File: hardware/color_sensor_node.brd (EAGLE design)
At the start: 27.9 x 27.9 mm, 20 parts, among them J1 JTAG, J2 JTAG, U1 ISL29125, U2 3.3V, U3 WS2811

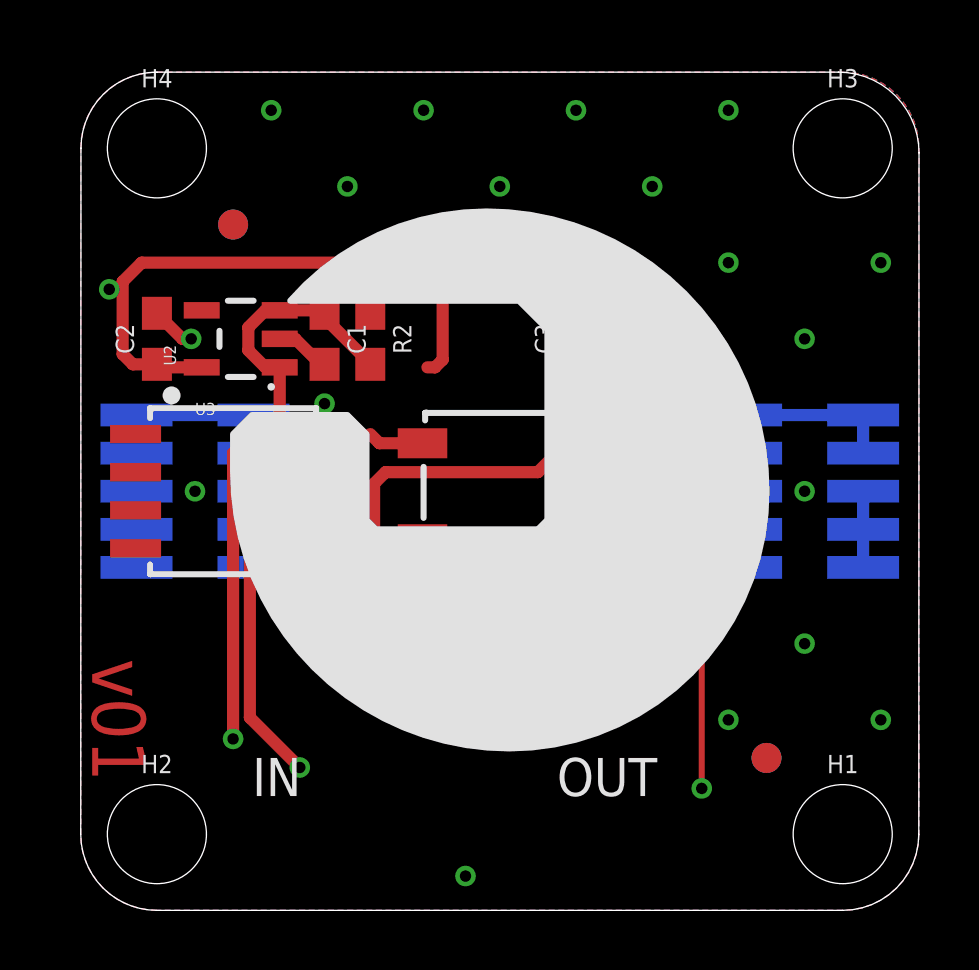
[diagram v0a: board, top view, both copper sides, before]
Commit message: idk
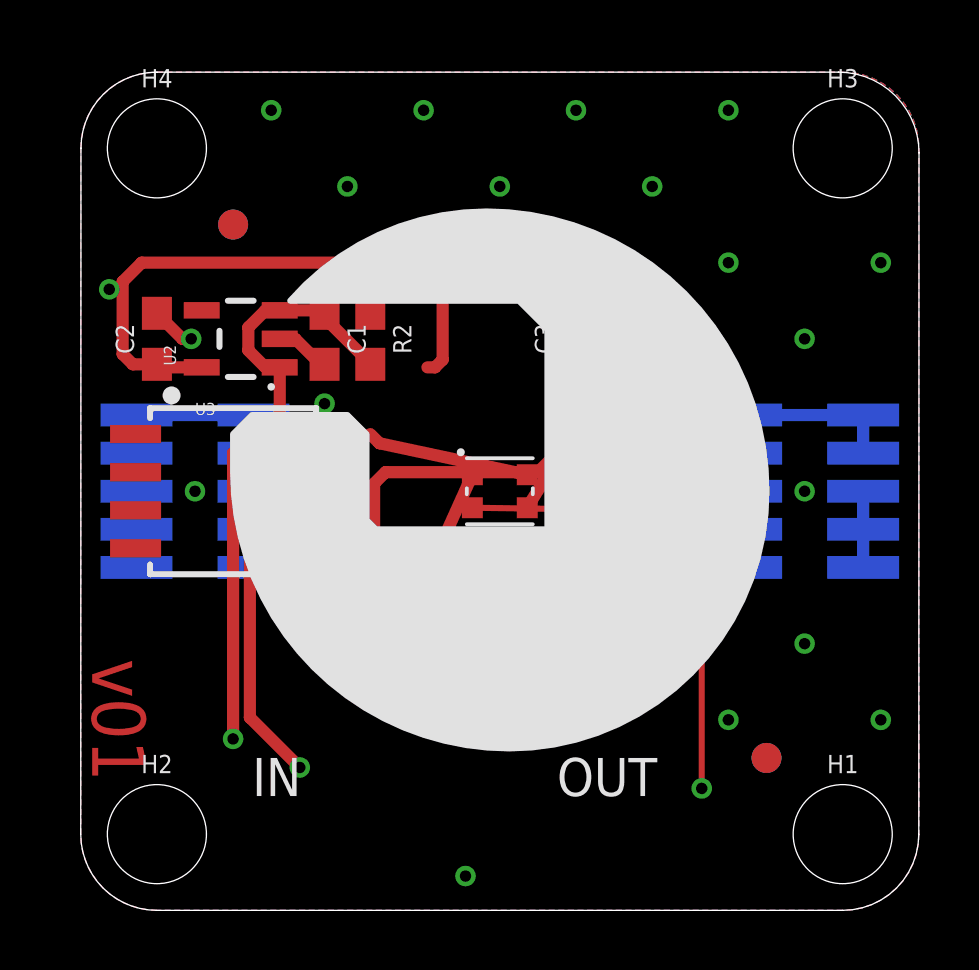
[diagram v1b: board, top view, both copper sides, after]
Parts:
- D1: device SparkFun-LED:WS2812B -> SparkFun-LED:WS2812-2020
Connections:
- net 5V: now also D1.4; no longer D1.1
- net DOUT: now also D1.1; no longer D1.2
- net GND: now also D1.2; no longer D1.3
- net N$4: now also D1.3; no longer D1.4
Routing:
- net 5V: track 27.7 -> 31.3 mm
- net DOUT: track 1.54 -> 4.05 mm
- net GND: track 16.5 -> 19.0 mm
- net N$4: track 10.7 -> 12.9 mm
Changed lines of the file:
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@@
 <attribute name="VALUE" x="3.302" y="19.05" size="0.6096" layer="27" font="vector" ratio="20" rot="R90" align="top-center"/>
 </element>
-<element name="D1" library="SparkFun-LED" package="WS2812B" value="WS2812B" x="13.97" y="13.97" rot="R180">
-<attribute name="PROD_ID" value="DIO-12503" x="13.97" y="13.97" size="1.778" layer="27" rot="R180" display="off"/>
-<attribute name="VALUE" value="WS2812B" x="13.97" y="13.97" size="1.778" layer="27" rot="R180" display="off"/>
+<element name="D1" library="SparkFun-LED" package="WS2812-2020" value="WS2812B" x="13.97" y="13.97" rot="R180">
 <attribute name="VALUE" x="13.97" y="16.764" size="0.6096" layer="27" font="vector" ratio="20" rot="R180" align="top-center"/>
 </element>
@@
 <contactref element="U1" pad="3"/>
 <contactref element="U3" pad="4"/>
-<contactref element="D1" pad="3"/>
+<contactref element="D1" pad="2"/>
 <wire x1="7.151" y1="19.05" x2="6.6341" y2="19.05" width="0.4064" layer="1"/>
 <wire x1="8.128" y1="18.2" x2="8.001" y2="18.2" width="0.4064" layer="1"/>
@@
 <via x="19.05" y="11.43" extent="1-16" drill="0.381"/>
 <wire x1="18.33" y1="13.47" x2="16.645" y2="13.47" width="0.2032" layer="1"/>
-<wire x1="16.547" y1="13.372" x2="16.547" y2="12.37" width="0.2032" layer="1"/>
+<wire x1="16.547" y1="13.372" x2="13.055" y2="13.42" width="0.2032" layer="1"/>
 <wire x1="16.645" y1="13.47" x2="16.547" y2="13.372" width="0.2032" layer="1"/>
 <wire x1="19.05" y1="24.13" x2="21.59" y2="26.67" width="0" layer="19" extent="1-1"/>
@@
 <wire x1="18.33" y1="13.47" x2="22.18" y2="16.51" width="0" layer="19" extent="1-16"/>
 <wire x1="19.05" y1="11.43" x2="18.33" y2="13.47" width="0" layer="19" extent="1-1"/>
-<wire x1="13.97" y1="11.43" x2="16.547" y2="12.37" width="0" layer="19" extent="1-1"/>
-<wire x1="16.51" y1="8.89" x2="16.547" y2="12.37" width="0" layer="19" extent="1-1"/>
+<wire x1="13.97" y1="11.43" x2="13.055" y2="13.42" width="0" layer="19" extent="1-1"/>
+<wire x1="16.51" y1="8.89" x2="13.055" y2="13.42" width="0" layer="19" extent="1-1"/>
 <wire x1="24.13" y1="8.89" x2="24.13" y2="13.97" width="0" layer="19" extent="1-1"/>
 <wire x1="26.67" y1="6.35" x2="24.13" y2="8.89" width="0" layer="19" extent="1-1"/>
@@
 <contactref element="U2" pad="3"/>
 <contactref element="C1" pad="1"/>
-<contactref element="D1" pad="1"/>
+<contactref element="D1" pad="4"/>
 <wire x1="8.028" y1="20" x2="6.6341" y2="20" width="0.4064" layer="1"/>
 <wire x1="8.128" y1="19.9" x2="8.028" y2="20" width="0.4064" layer="1"/>
@@
 <wire x1="6.6341" y1="15.9051" x2="6.604" y2="15.875" width="0.4064" layer="1"/>
 <wire x1="6.6341" y1="18.1" x2="6.6341" y2="15.9051" width="0.4064" layer="1"/>
-<wire x1="9.957" y1="15.57" x2="11.393" y2="15.57" width="0.4064" layer="1"/>
+<wire x1="9.957" y1="15.57" x2="14.885" y2="14.52" width="0.4064" layer="1"/>
 <wire x1="9.652" y1="15.875" x2="9.957" y2="15.57" width="0.4064" layer="1"/>
 <contactref element="U3" pad="8"/>
 <via x="5.08" y="5.715" extent="1-16" drill="0.381"/>
 <wire x1="26.08" y1="13.97" x2="22.18" y2="15.24" width="0" layer="19" extent="16-16"/>
-<wire x1="11.393" y1="15.57" x2="22.18" y2="15.24" width="0" layer="19" extent="1-16"/>
+<wire x1="14.885" y1="14.52" x2="22.18" y2="15.24" width="0" layer="19" extent="1-16"/>
 <wire x1="8.3312" y1="15.875" x2="9.652" y2="15.875" width="0" layer="19" extent="1-1"/>
 <wire x1="6.6341" y1="15.9051" x2="8.3312" y2="15.875" width="0" layer="19" extent="1-1"/>
@@
 </signal>
 <signal name="DOUT">
-<contactref element="D1" pad="2"/>
+<contactref element="D1" pad="1"/>
 <contactref element="J2" pad="6"/>
-<wire x1="11.393" y1="10.832" x2="11.393" y2="12.37" width="0.4064" layer="1"/>
+<wire x1="11.393" y1="10.832" x2="13.055" y2="14.52" width="0.4064" layer="1"/>
 <via x="11.393" y="10.832" extent="1-16" drill="0.381"/>
 <wire x1="11.393" y1="10.832" x2="22.18" y2="13.97" width="0" layer="19" extent="1-16"/>
 </signal>
 <signal name="N$4">
-<contactref element="D1" pad="4"/>
+<contactref element="D1" pad="3"/>
 <contactref element="U3" pad="5"/>
 <wire x1="9.398" y1="12.065" x2="8.3312" y2="12.065" width="0.4064" layer="1"/>
 <wire x1="9.779" y1="12.446" x2="9.398" y2="12.065" width="0.4064" layer="1"/>
-<wire x1="16.547" y1="15.57" x2="16.205" y2="15.57" width="0.4064" layer="1"/>
+<wire x1="14.885" y1="13.42" x2="16.205" y2="15.57" width="0.4064" layer="1"/>
 <wire x1="15.24" y1="14.605" x2="10.16" y2="14.605" width="0.4064" layer="1"/>
 <wire x1="10.16" y1="14.605" x2="9.779" y2="14.224" width="0.4064" layer="1"/>
